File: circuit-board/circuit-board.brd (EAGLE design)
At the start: 100 x 80 mm, 51 parts, among them IC1 UA78M05DCY, Q1 BC547B, Q2 BC547B, U1 MAX3232, U2 ATMEGA328P_TQFP, U3 ADUM1201BRZ, Y2 16MHz

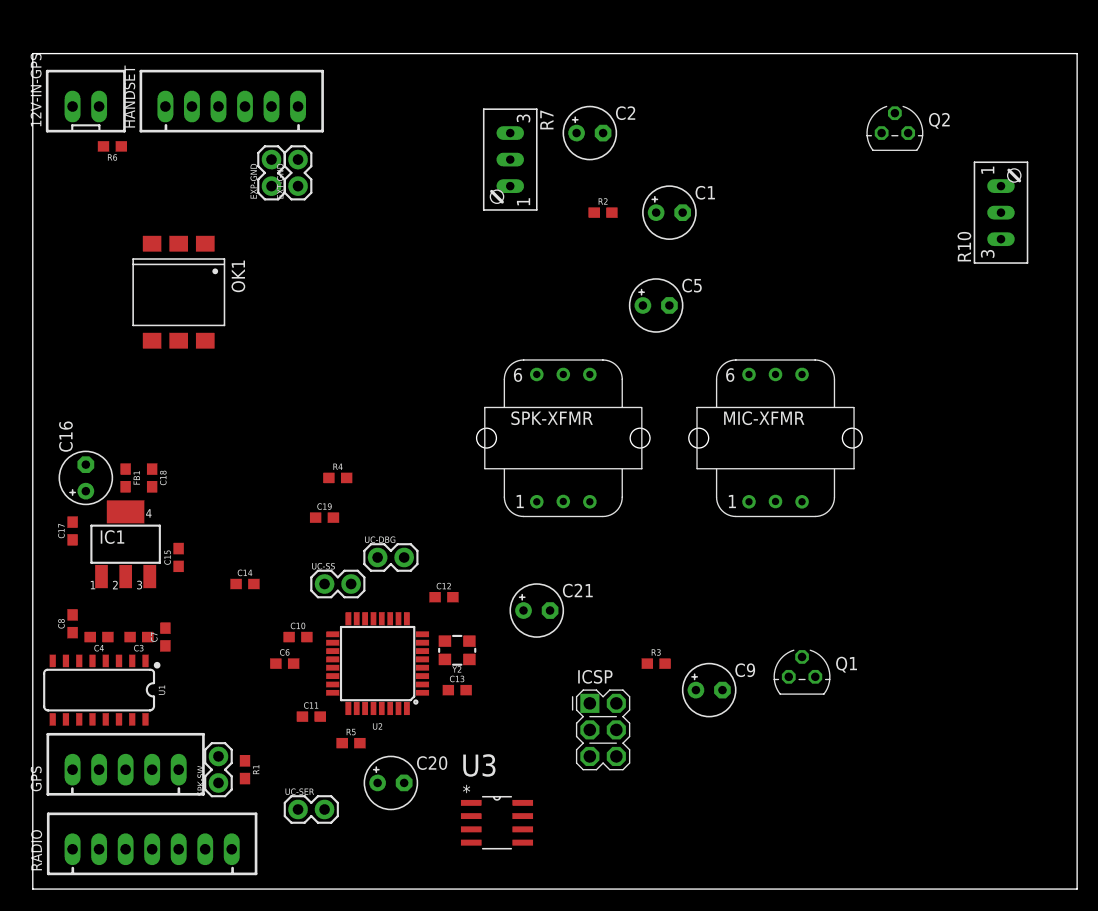
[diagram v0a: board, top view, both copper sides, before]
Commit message: Lay out circuit board, preliminary
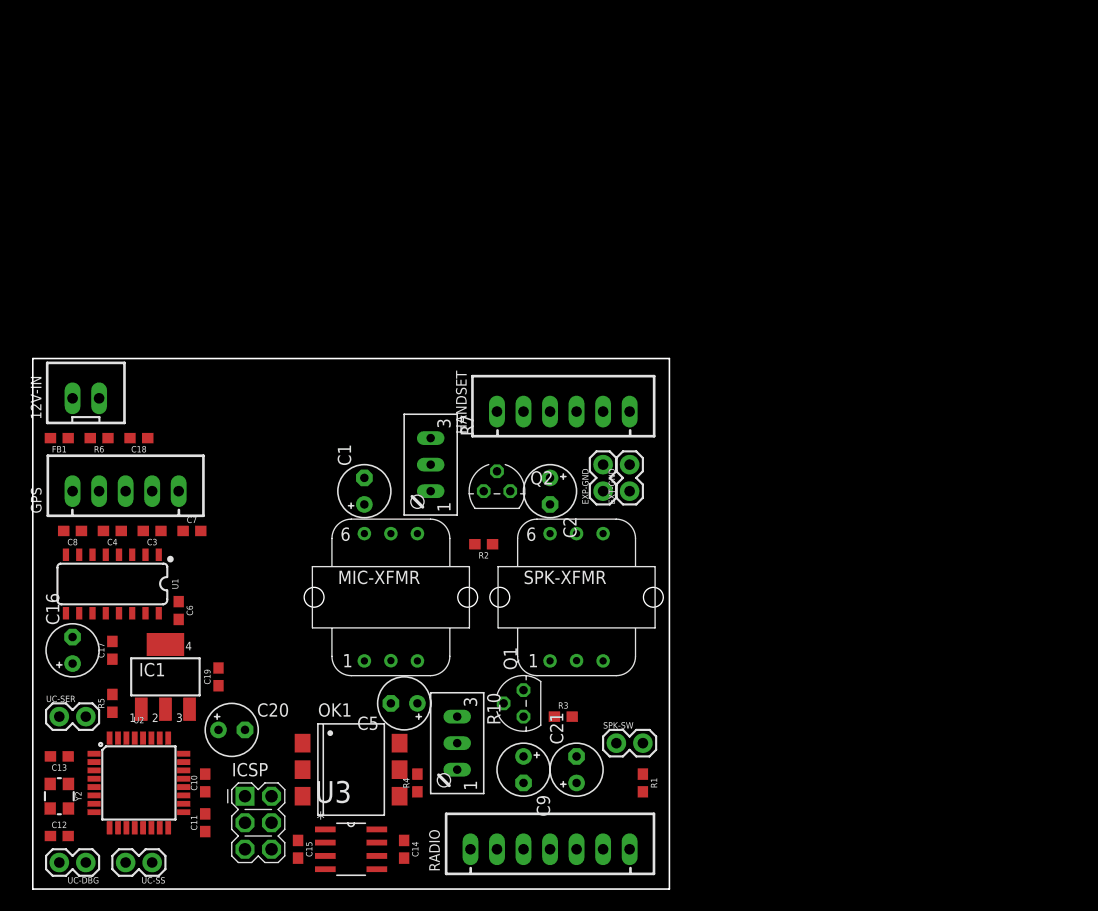
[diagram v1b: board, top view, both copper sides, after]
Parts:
- removed 12V-IN-GPS: JST-XH-02-PIN-LONG-PAD, Rembrandt Electronics - JST XH Connectors v1-0:JST-XH-02-PACKAGE-LONG-PAD
- added 12V-IN: JST-XH-02-PIN-LONG-PAD, Rembrandt Electronics - JST XH Connectors v1-0:JST-XH-02-PACKAGE-LONG-PAD
- moved R10 74.6 mm to (39.4, 14.0), turned to 270 degrees
- moved Q2 51.3 mm to (44.5, 38.1)
- moved OK1 48.6 mm to (30.5, 11.4), turned to 270 degrees
- moved C5 45.1 mm to (35.6, 17.8), turned to 180 degrees
- moved C12 43.3 mm to (2.54, 5.08)
- moved EXP-GND 43.1 mm to (54.6, 38.1)
- moved EXT-GND 43.1 mm to (57.1, 38.1)
- moved HANDSET 43.1 mm to (50.8, 45.7)
- moved Y2 40.6 mm to (2.54, 8.89), turned to 270 degrees
- moved UC-DBG 40.4 mm to (5.08, 2.54), turned to 180 degrees
- moved MIC-XFMR 39.9 mm to (34.3, 27.9)
- moved C1 39.6 mm to (31.8, 38.1), turned to 90 degrees
- moved C13 38.6 mm to (2.54, 12.7), turned to 180 degrees
- moved SPK-SW 38.3 mm to (55.9, 14.0), turned to 0 degrees
- moved R1 38.1 mm to (58.4, 10.2)
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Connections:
- net 12V: now also 12V-IN.2; no longer 12V-IN-GPS.2
- net GNDA: now also 12V-IN.1; no longer 12V-IN-GPS.1
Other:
- board size 100 x 80 mm -> 61 x 50.8 mm

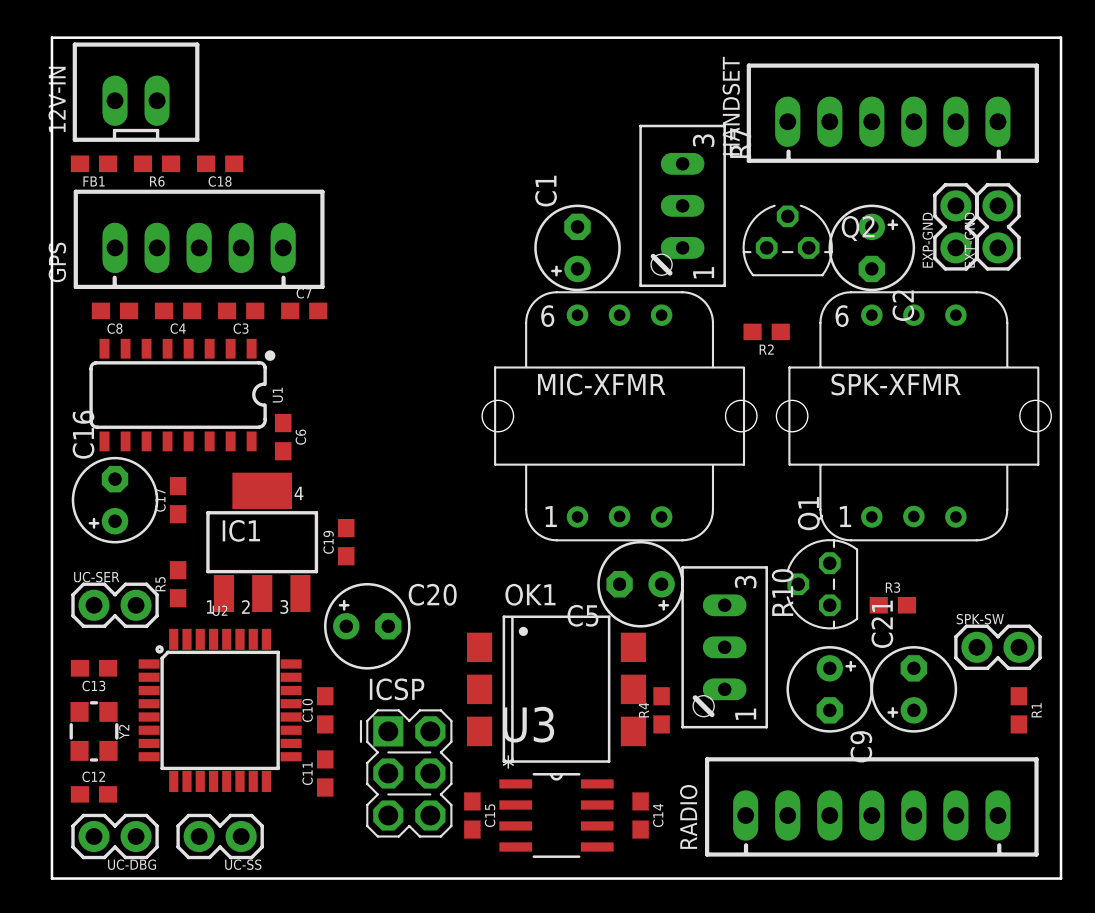
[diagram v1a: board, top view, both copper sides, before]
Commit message: Minimize V2 board layout
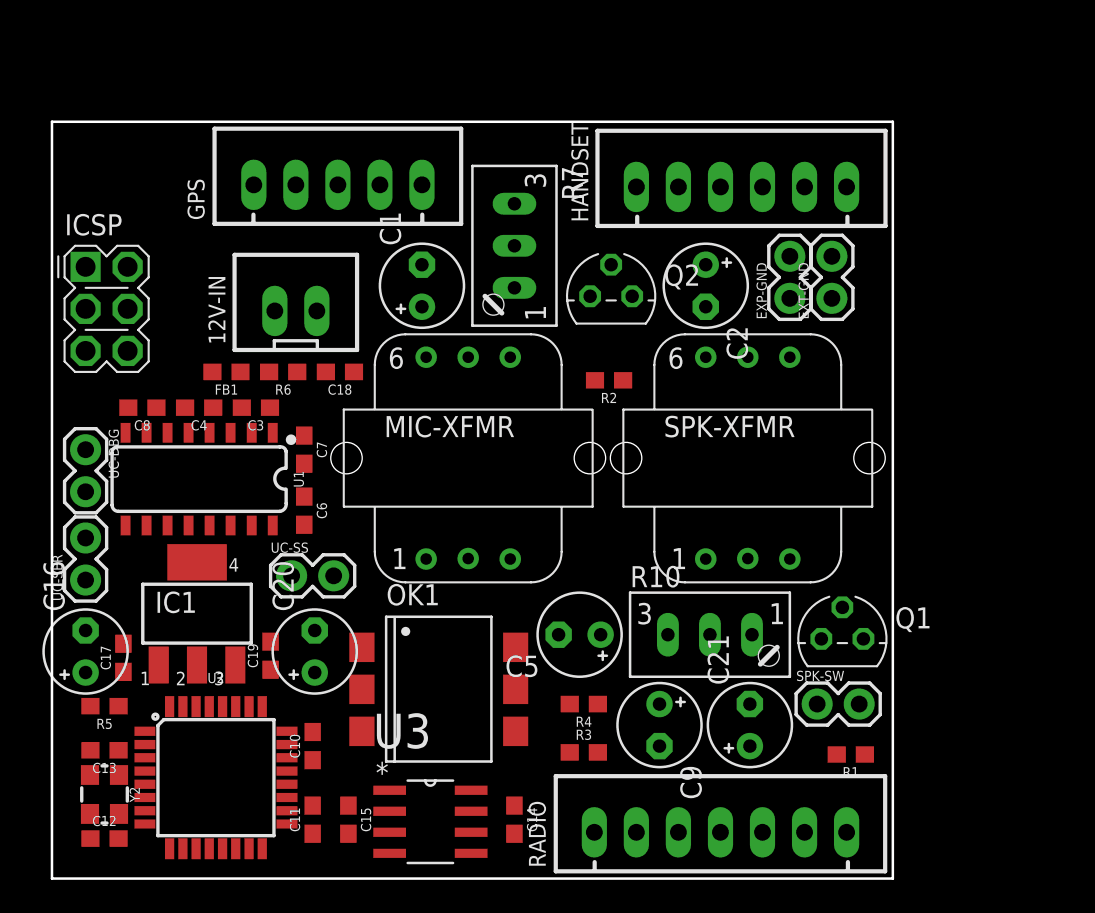
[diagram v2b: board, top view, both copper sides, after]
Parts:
- moved ICSP 33.5 mm to (2.03, 37.0)
- moved UC-DBG 23.6 mm to (2.03, 25.9), turned to 270 degrees
- moved R3 20.7 mm to (32.1, 7.62)
- moved UC-SS 16.0 mm to (14.5, 18.3), turned to 0 degrees
- moved 12V-IN 16.0 mm to (14.7, 34.3)
- moved FB1 14.9 mm to (10.5, 30.6)
- moved R6 14.7 mm to (14.0, 30.6)
- moved C18 14.5 mm to (17.4, 30.6)
- moved Q2 11.1 mm to (33.8, 35.2)
- moved C9 10.5 mm to (36.7, 9.27)
- moved R1 10.5 mm to (48.3, 7.49), turned to 180 degrees
- moved EXP-GND 10.5 mm to (44.6, 35.1)
- moved EXT-GND 10.5 mm to (47.1, 35.1)
- moved R7 10.4 mm to (26.7, 38.2)
- moved SPK-XFMR 10.3 mm to (42.0, 25.4)
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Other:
- board size 61 x 50.8 mm -> 50.8 x 45.7 mm
